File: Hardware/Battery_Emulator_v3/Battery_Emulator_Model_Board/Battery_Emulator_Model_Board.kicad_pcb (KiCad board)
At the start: 2 copper layers, 43 parts, among them J1 Vin, J10 Conn_01x05, J11 Conn_01x05, J12 Conn_01x05, J13 Conn_01x05, J14 Conn_01x05, J15 Conn_01x05, J16 Conn_01x05, J17 Conn_01x05, J2 USB4105-GF-A-060, J3 Conn_01x05, J5 Conn_01x05, J6 Conn_01x05, J7 Conn_01x05, J8 Conn_01x05, J9 Conn_01x05, U1 ATmega328PB-A, U2 KA78M05_TO252, U3 FT230XS-R, U4 74AHC2G125DP,125, Y1 Crystal_GND24

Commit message: Hardware Update
Updated the v3 model board PCB layout.
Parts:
- moved J10 307.6 mm to (323.9, 118.9), turned to -90 degrees
- moved J11 289.7 mm to (324.6, 97.0)
- moved J9 278.2 mm to (279.7, 118.9), turned to -90 degrees
- moved J17 261.0 mm to (313.7, 86.3), turned to 90 degrees
- moved J16 230.6 mm to (269.5, 86.3), turned to 90 degrees
- moved J15 200.3 mm to (225.3, 86.3), turned to 90 degrees
- moved J8 195.3 mm to (235.4, 118.9), turned to -90 degrees
- moved J14 170.4 mm to (181.3, 86.3), turned to 90 degrees
- moved J7 170.0 mm to (191.4, 118.9), turned to -90 degrees
- moved J6 146.8 mm to (147.4, 118.9), turned to -90 degrees
- moved J5 126.7 mm to (103.4, 118.9), turned to -90 degrees
- moved J3 112.0 mm to (60.4, 118.9), turned to -90 degrees
- moved J13 87.6 mm to (137.3, 86.3), turned to 90 degrees
- moved J12 66.7 mm to (93.3, 86.3), turned to 90 degrees
- moved TP3 61.0 mm to (77.1, 100.8)
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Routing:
- net +5V: track 27.6 -> 595.8 mm, vias 0 -> 2
- net +12V: track 13.1 -> 527.4 mm, vias 0 -> 12
- net /SCL: track 2.88 -> 480.5 mm, vias 0 -> 1
- net /SDA_cell_8-14: track 0.00 -> 338.0 mm, vias 0 -> 2
- net /SDA_cell_1-7: track 0.00 -> 335.4 mm, vias 0 -> 2
- net /TX: track 0.00 -> 14.7 mm, vias 0 -> 2
- net /RX: track 0.00 -> 12.9 mm, vias 0 -> 2
- net /SDA: track 6.93 -> 13.2 mm, vias 0 -> 2
- net GND: track 7.30 -> 8.62 mm, vias 0 -> 1
- added copper zone on B.Cu, net GND

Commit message: Hardware Update
Finished the Model Board PCB
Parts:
- added TP4: GND, TestPoint:TestPoint_Pad_D2.5mm, F.Cu at (80.8, 100.8)
- moved H4 199.8 mm to (305.2, 113.8)
- moved H3 195.9 mm to (305.2, 94.2)
- moved H2 94.7 mm to (85.0, 113.8)
- moved H1 83.9 mm to (85.0, 94.2)
- moved J12 2.87 mm to (93.3, 89.2)
- moved J13 2.87 mm to (137.3, 89.2)
- moved J14 2.87 mm to (181.3, 89.2)
- moved J15 2.87 mm to (225.3, 89.2)
- moved J16 2.87 mm to (269.5, 89.2)
- moved J17 2.87 mm to (313.7, 89.2)
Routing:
- net +12V: track 527.4 -> 569.1 mm, vias 12 -> 13
- net /SCL: track 480.5 -> 463.3 mm, vias 1 -> 38
- net /SDA_cell_8-14: track 338.0 -> 322.5 mm
- net +5V: track 595.8 -> 610.0 mm, vias 2 -> 6
- net GND: track 8.62 -> 10.9 mm, vias 1 -> 36
- net /SDA_cell_1-7: track 335.4 -> 337.2 mm
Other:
- board outline added: 278.4 x 38.2 mm

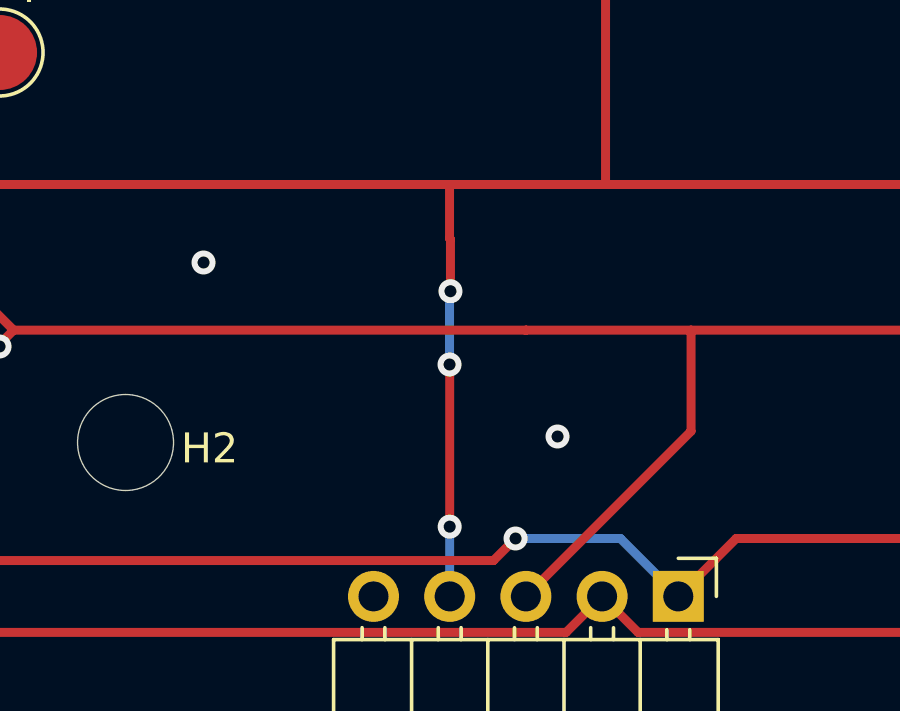
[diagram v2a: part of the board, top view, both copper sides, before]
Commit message: Hardware update
updated the model board pcb and the cell pcb
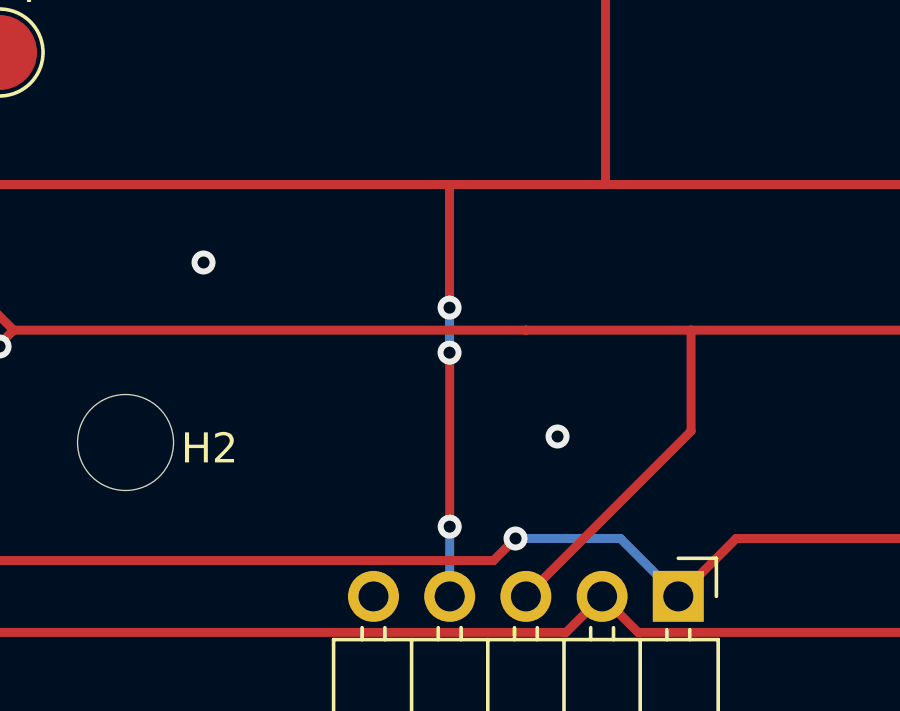
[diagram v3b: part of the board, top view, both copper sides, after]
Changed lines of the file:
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@@
   (segment (start 71.2 120.2) (end 80.8 110.6) (width 0.3) (layer "B.Cu") (net 7))
   (segment (start 64.6 102.8925) (end 64.6 103.6055) (width 0.3) (layer "F.Cu") (net 8))
-  (segment (start 95.8 107) (end 95.8 105.2) (width 0.3) (layer "F.Cu") (net 8))
   (segment (start 66.15 101.605) (end 66.15 100.805) (width 0.3) (layer "F.Cu") (net 8))
   (segment (start 189 105.2) (end 227.8 105.2) (width 0.3) (layer "F.Cu") (net 8))
   (segment (start 316.4 105.2) (end 319.360953 105.2) (width 0.3) (layer "F.Cu") (net 8))
-  (segment (start 95.805 116.605) (end 95.805 111.205) (width 0.3) (layer "F.Cu") (net 8))
   (segment (start 232.8 91.9495) (end 232.8 96.6505) (width 0.3) (layer "F.Cu") (net 8))
   (segment (start 272 105.2) (end 277 105.2) (width 0.3) (layer "F.Cu") (net 8))
+  (segment (start 95.8 110.8045) (end 95.805 110.8095) (width 0.3) (layer "F.Cu") (net 8))
   (segment (start 232.8 98.1495) (end 232.8 105.2) (width 0.3) (layer "F.Cu") (net 8))
   (segment (start 319.360953 105.2) (end 319.361327 105.199626) (width 0.3) (layer "F.Cu") (net 8))
-  (segment (start 95.805 111.205) (end 95.8 111.2) (width 0.3) (layer "F.Cu") (net 8))
   (segment (start 316.4 115.4) (end 316.4 105.2) (width 0.3) (layer "F.Cu") (net 8))
   (segment (start 321.6 100.119954) (end 321.6 105.2) (width 0.3) (layer "F.Cu") (net 8))
@@
   (segment (start 101 91.9495) (end 101 96.6505) (width 0.3) (layer "F.Cu") (net 8))
   (segment (start 183.6 105.2) (end 189 105.2) (width 0.3) (layer "F.Cu") (net 8))
-  (segment (start 95.83034 107.03034) (end 95.8 107) (width 0.3) (layer "F.Cu") (net 8))
   (segment (start 139.8 109.3055) (end 139.8 105.2) (width 0.3) (layer "F.Cu") (net 8))
-  (segment (start 95.83034 108.757585) (end 95.83034 107.03034) (width 0.3) (layer "F.Cu") (net 8))
   (segment (start 321.570023 97.970069) (end 321.599977 98.000023) (width 0.3) (layer "F.Cu") (net 8))
   (segment (start 227.8 109.3055) (end 227.8 105.2) (width 0.3) (layer "F.Cu") (net 8))
@@
   (segment (start 189 98.1495) (end 189 105.2) (width 0.3) (layer "F.Cu") (net 8))
   (segment (start 321.540023 100.059977) (end 321.6 100.119954) (width 0.3) (layer "F.Cu") (net 8))
+  (segment (start 95.8 109.3055) (end 95.8 105.2) (width 0.3) (layer "F.Cu") (net 8))
   (segment (start 64.8625 102.8925) (end 66.15 101.605) (width 0.3) (layer "F.Cu") (net 8))
   (segment (start 272 116.2505) (end 272 110.8045) (width 0.3) (layer "F.Cu") (net 8))
   (segment (start 145 98.1495) (end 145 105.2) (width 0.3) (layer "F.Cu") (net 8))
+  (segment (start 95.805 110.8095) (end 95.805 116.605) (width 0.3) (layer "F.Cu") (net 8))
   (via (at 189 98.1495) (size 0.8) (drill 0.4) (layers "F.Cu" "B.Cu") (net 8))
   (via (at 321.629977 92.970023) (size 0.8) (drill 0.4) (layers "F.Cu" "B.Cu") (net 8))
@@
   (via (at 277 96.6505) (size 0.8) (drill 0.4) (layers "F.Cu" "B.Cu") (net 8))
   (via (at 183.8 109.3055) (size 0.8) (drill 0.4) (layers "F.Cu" "B.Cu") (net 8))
-  (via (at 95.8 111.2) (size 0.8) (drill 0.4) (layers "F.Cu" "B.Cu") (net 8))
+  (via (at 95.8 110.8045) (size 0.8) (drill 0.4) (layers "F.Cu" "B.Cu") (net 8))
   (via (at 227.8 110.8045) (size 0.8) (drill 0.4) (layers "F.Cu" "B.Cu") (net 8))
   (via (at 321.570023 95.029977) (size 0.8) (drill 0.4) (layers "F.Cu" "B.Cu") (net 8))
@@
   (via (at 277.2 91.9495) (size 0.8) (drill 0.4) (layers "F.Cu" "B.Cu") (net 8))
   (via (at 227.8 109.3055) (size 0.8) (drill 0.4) (layers "F.Cu" "B.Cu") (net 8))
-  (via (at 95.83034 108.757585) (size 0.8) (drill 0.4) (layers "F.Cu" "B.Cu") (net 8))
+  (via (at 95.8 109.3055) (size 0.8) (drill 0.4) (layers "F.Cu" "B.Cu") (net 8))
   (via (at 101 98.1495) (size 0.8) (drill 0.4) (layers "F.Cu" "B.Cu") (net 8))
   (via (at 321.6 105.2) (size 0.8) (drill 0.4) (layers "F.Cu" "B.Cu") (net 8))
@@
   (segment (start 95.805 118.93) (end 95.805 116.605) (width 0.3) (layer "B.Cu") (net 8))
   (segment (start 227.805 116.2555) (end 227.8 116.2505) (width 0.3) (layer "B.Cu") (net 8))
+  (segment (start 95.8 109.3055) (end 95.8 110.8045) (width 0.3) (layer "B.Cu") (net 8))
   (segment (start 100.895 89.175) (end 100.895 91.8445) (width 0.3) (layer "B.Cu") (net 8))
   (segment (start 316.27 118.93) (end 316.27 115.53) (width 0.3) (layer "B.Cu") (net 8))
@@
   (segment (start 272.055 116.3055) (end 272 116.2505) (width 0.3) (layer "B.Cu") (net 8))
   (segment (start 139.8 110.8045) (end 139.8 109.3055) (width 0.3) (layer "B.Cu") (net 8))
-  (segment (start 95.8 111.2) (end 95.8 108.787925) (width 0.3) (layer "B.Cu") (net 8))
   (segment (start 183.805 118.93) (end 183.805 116.2555) (width 0.3) (layer "B.Cu") (net 8))
   (segment (start 321.6 105.2) (end 322.2 104.6) (width 0.3) (layer "B.Cu") (net 8))
@@
   (segment (start 145 96.6505) (end 145 98.1495) (width 0.3) (layer "B.Cu") (net 8))
   (segment (start 272.055 118.93) (end 272.055 116.3055) (width 0.3) (layer "B.Cu") (net 8))
-  (segment (start 95.8 108.787925) (end 95.83034 108.757585) (width 0.3) (layer "B.Cu") (net 8))
   (segment (start 139.805 116.2555) (end 139.8 116.2505) (width 0.3) (layer "B.Cu") (net 8))
   (segment (start 321.629977 92.970023) (end 321.629977 94.970023) (width 0.3) (layer "B.Cu") (net 8))
